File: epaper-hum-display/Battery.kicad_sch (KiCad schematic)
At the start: 48 parts, among them J3 USB_C_Receptacle, Q2 PMV65XP,215, U2 TPS25750S, U3 BQ25798, U4 CDSOT23-0502B, U5 CDSOT23-0502B, U6 SISF00DN, U7 TPS7A2018PDBVR, U8 TPS7A2033PDBVR

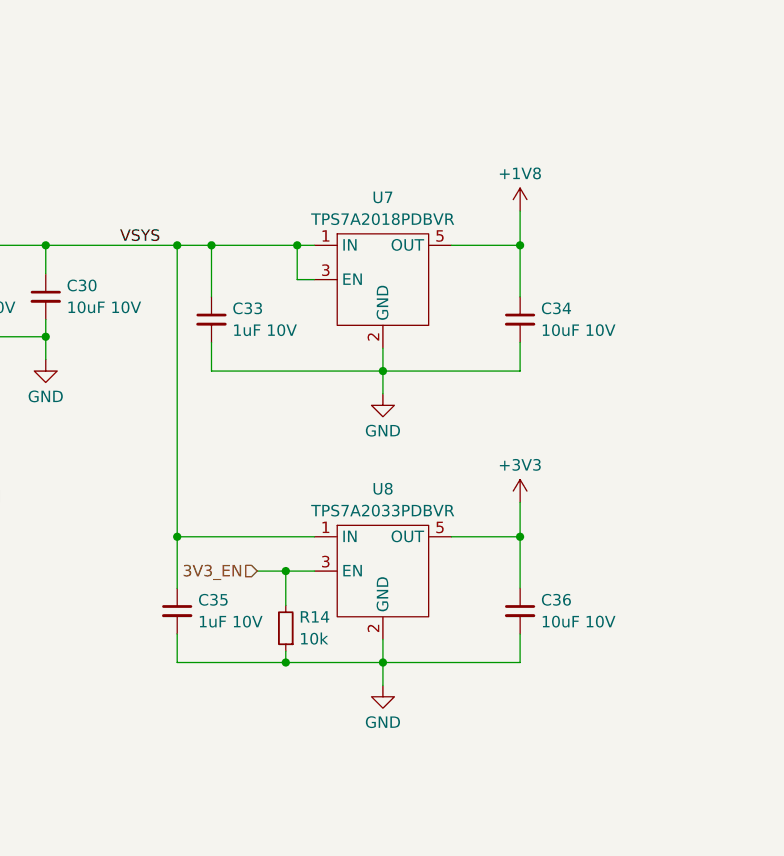
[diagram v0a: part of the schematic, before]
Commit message: WIP
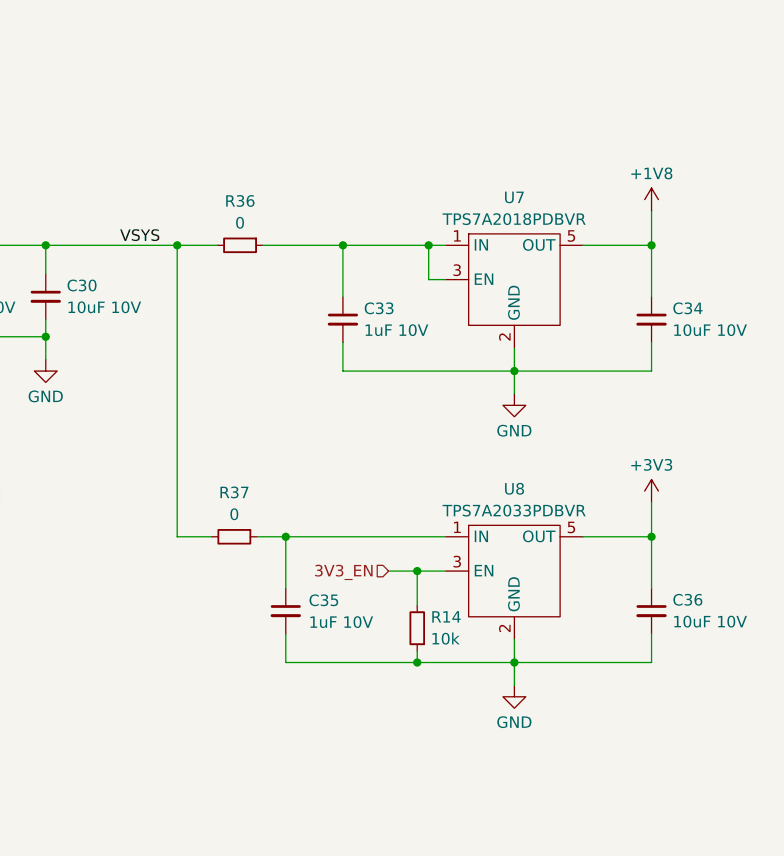
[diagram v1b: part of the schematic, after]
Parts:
- added R36, R37: 0, Resistor_SMD:R_0805_2012Metric, symbol Device:R_Small
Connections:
- net VSYS: now also R36.2, R37.2; no longer C33.1, C35.1, U7.1 (IN), U7.3 (EN), U8.1 (IN)
- new net: C35.1, R37.1, U8.1 (IN)
- new net: C33.1, R36.1, U7.1 (IN), U7.3 (EN)
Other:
- moved on the sheet: C33, C34, C35, C36, R14, U7, U8
